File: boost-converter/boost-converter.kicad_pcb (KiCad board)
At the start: 2 copper layers, 18 parts, among them P1 CONN_02X01, P2 CONN_02X01, Q1 IRF730, Q2 BC547, U1 NE555

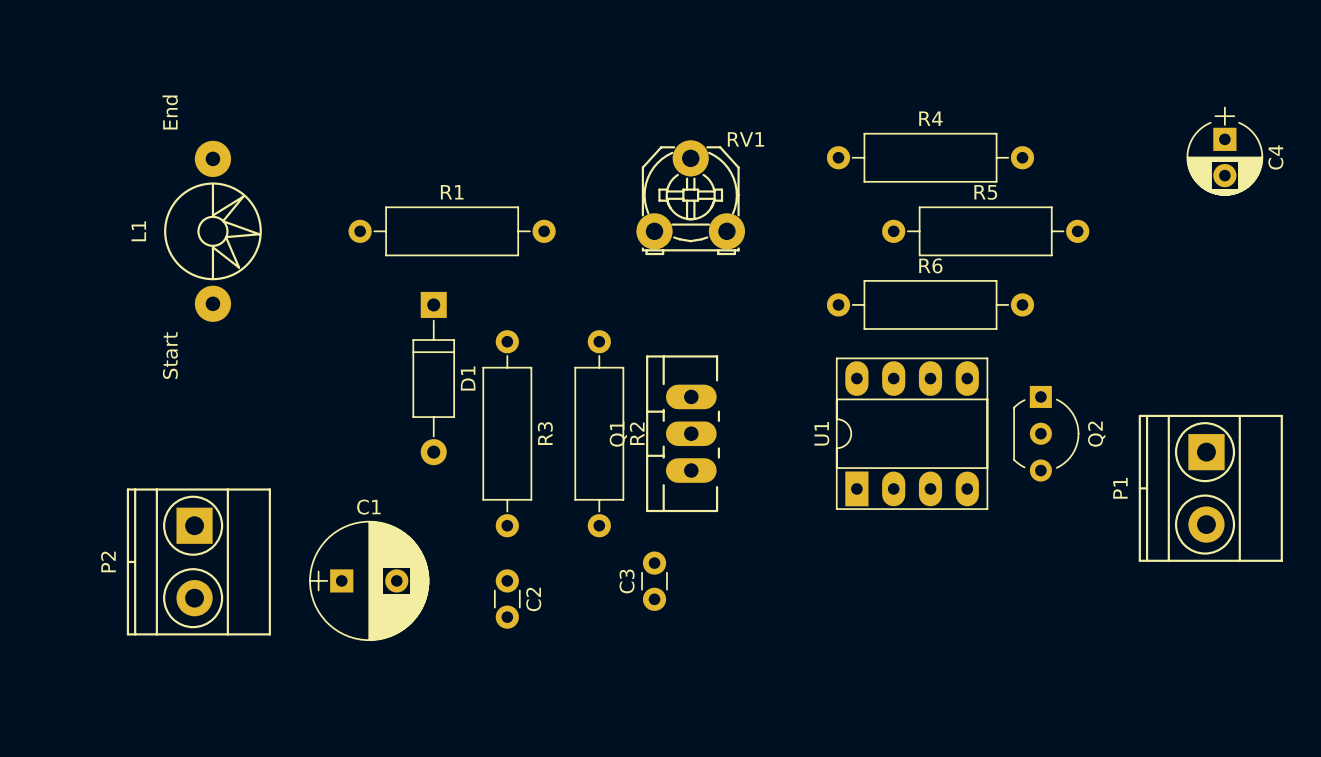
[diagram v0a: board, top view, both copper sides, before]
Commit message: Dokończone pcb + pdf
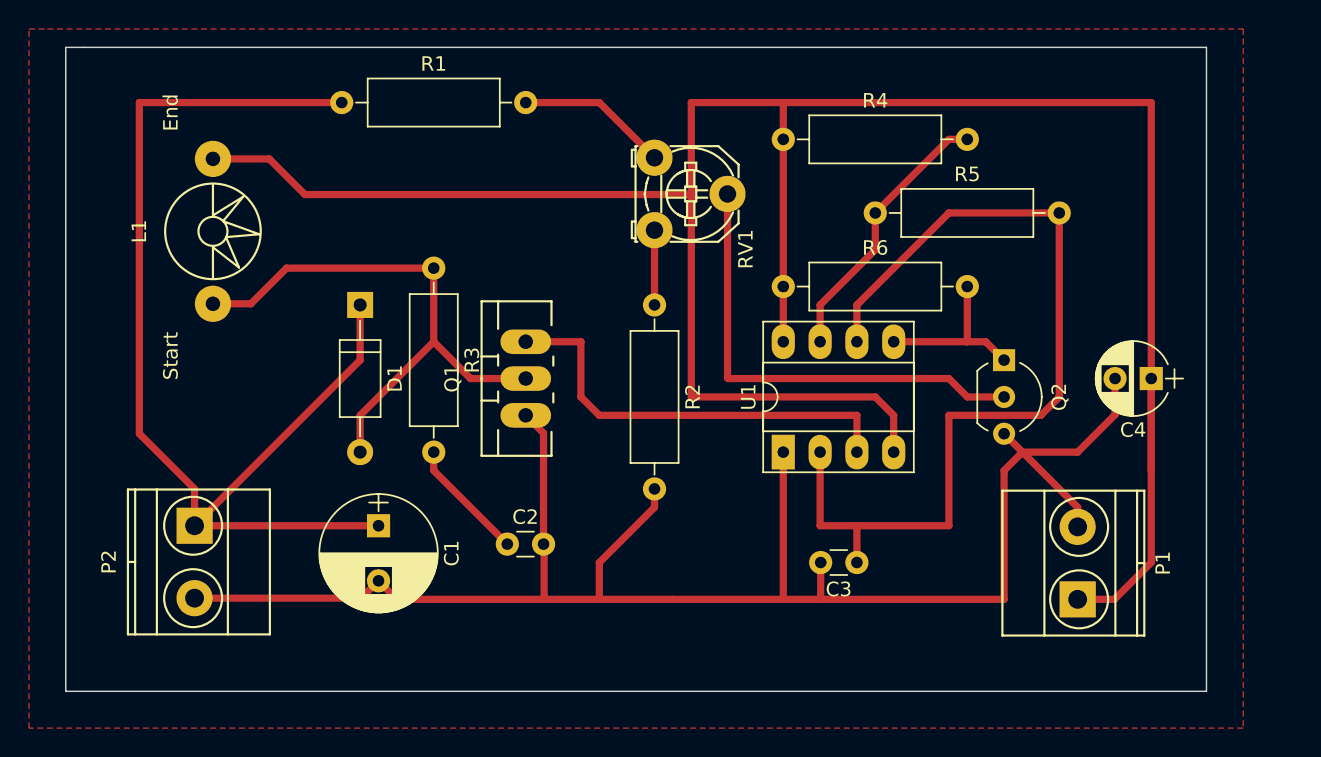
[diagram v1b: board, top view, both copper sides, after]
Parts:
- moved C4 17.3 mm to (102.9, 80.0), turned to 180 degrees
- moved C3 14.2 mm to (82.5, 92.7), turned to 180 degrees
- moved P1 13.5 mm to (97.8, 95.2), turned to 90 degrees
- moved Q1 12.0 mm to (59.7, 80.0)
- moved R1 8.98 mm to (47.0, 61.0)
- moved R3 7.18 mm to (53.3, 72.4)
- moved U1 5.68 mm to (77.5, 85.1)
- moved D1 5.08 mm to (48.3, 74.9)
- moved RV1 5.08 mm to (68.6, 64.8), turned to 270 degrees
- moved C1 4.58 mm to (49.5, 90.2), turned to 270 degrees
- moved R2 4.58 mm to (68.6, 74.9)
- moved R6 4.02 mm to (77.5, 73.7)
- moved R4 4.02 mm to (77.5, 63.5)
- moved Q2 3.59 mm to (92.7, 78.7)
- moved C2 2.54 mm to (58.4, 91.4), turned to 0 degrees
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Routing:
- net +9V: track 0.00 -> 164.0 mm
- net Earth: track 0.00 -> 121.3 mm
- net VSSA: track 0.00 -> 77.4 mm
- net Net-(C3-Pad1): track 0.00 -> 64.1 mm
- net Net-(D1-Pad2): track 0.00 -> 38.5 mm
- net Net-(Q2-Pad2): track 0.00 -> 32.3 mm
- net Net-(Q1-Pad3): track 0.00 -> 29.7 mm
- net Net-(R4-Pad2): track 0.00 -> 18.9 mm
- net Net-(Q2-Pad1): track 0.00 -> 12.0 mm
- net Net-(R1-Pad2): track 0.00 -> 10.5 mm
- net Net-(C2-Pad1): track 0.00 -> 8.45 mm
- net Net-(R2-Pad1): track 0.00 -> 5.16 mm
- added copper zone on F.Cu, net Earth
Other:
- board outline added: 78.7 x 44.4 mm
- net class Default: trace_width 0.25 -> 0.5
- rule trace_min: 0.2 -> 0.3
